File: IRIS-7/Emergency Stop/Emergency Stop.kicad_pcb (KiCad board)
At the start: 2 copper layers, 40 x 50 mm, 36 parts, among them IC1 LMR16006, J1 5mm TB, J2 ESTOP, J3 Pwr, J4 5mm TB, Q1 BSS123, Q2 BSS123, Q3 DMP3099L

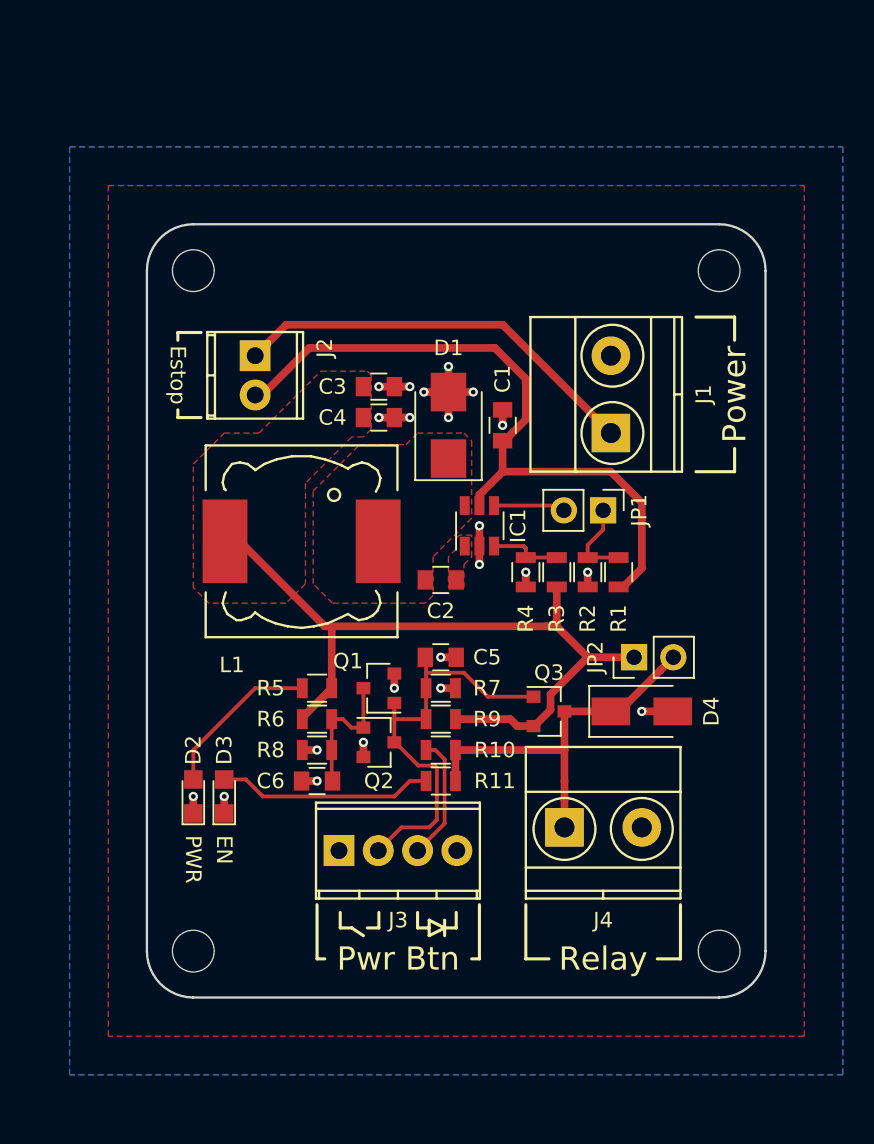
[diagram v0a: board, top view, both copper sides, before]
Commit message: Finalize board design for Rev A release
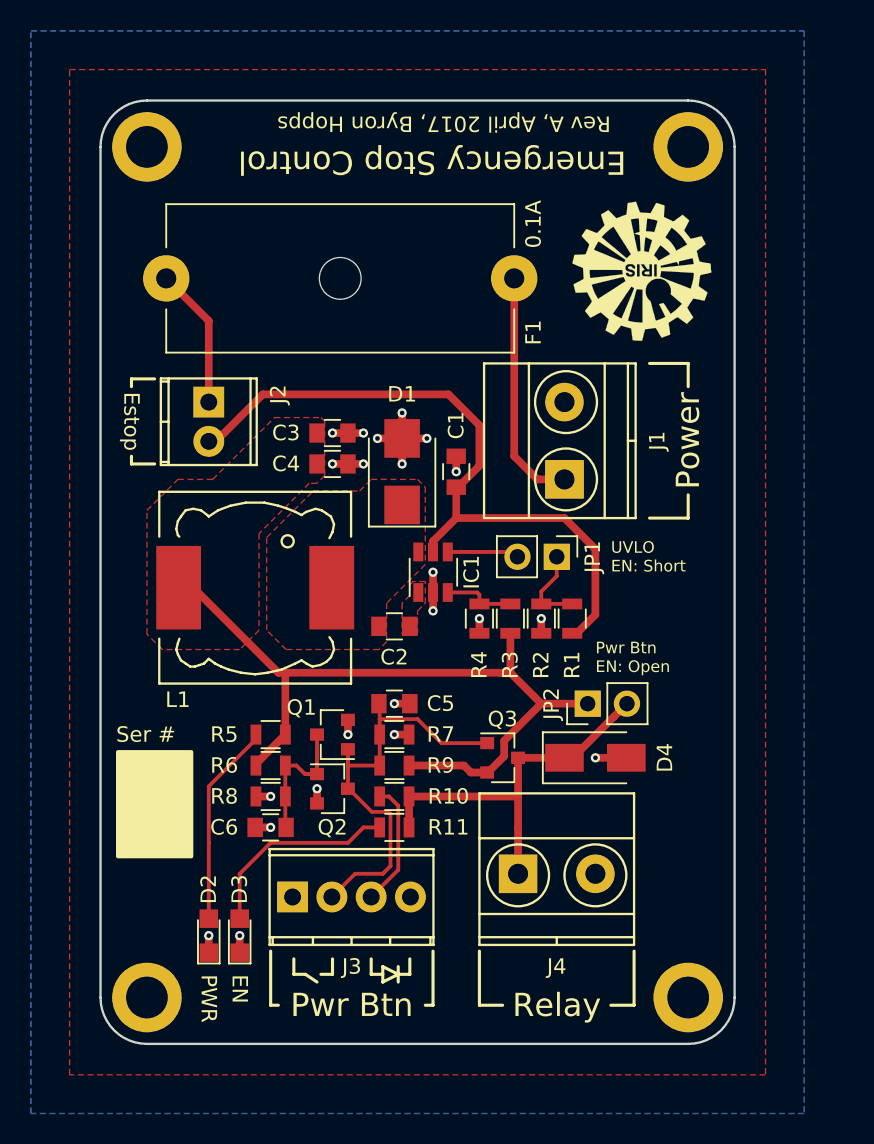
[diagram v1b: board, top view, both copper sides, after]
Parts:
- removed the REF** at (137.0, 97.0)
- removed the REF** at (103.0, 97.0)
- removed the REF** at (103.0, 53.0)
- removed the REF** at (137.0, 53.0)
- added F1: F, Fuse_Holders_and_Fuses:Fuseholder5x20_horiz_open_Schurter_0031_8201, F.Cu at (123.8, 53.5)
- added G***: LOGO, IRIS_Logos:IRIS_Logo_9.2, F.Cu at (132.0, 53.0)
- added REF**: MountingHole_2.7mm_M2.5_ISO7380_Pad, Mounting_Holes:MountingHole_2.7mm_M2.5_ISO7380_Pad, F.Cu at (100.0, 100.0)
- added REF**: MountingHole_2.7mm_M2.5_ISO7380_Pad, Mounting_Holes:MountingHole_2.7mm_M2.5_ISO7380_Pad, F.Cu at (135.0, 100.0)
- added REF**: MountingHole_2.7mm_M2.5_ISO7380_Pad, Mounting_Holes:MountingHole_2.7mm_M2.5_ISO7380_Pad, F.Cu at (135.0, 45.0)
- added REF**: MountingHole_2.7mm_M2.5_ISO7380_Pad, Mounting_Holes:MountingHole_2.7mm_M2.5_ISO7380_Pad, F.Cu at (100.0, 45.0)
- JP1, JP2: footprint Socket_Strips:Socket_Strip_Straight_1x02_Pitch2.54mm -> Pin_Headers:Pin_Header_Straight_1x02_Pitch2.54mm
- moved D2 9.06 mm to (104.0, 96.0)
- moved D3 9.06 mm to (106.0, 96.0)
- moved C1 4.24 mm to (120.0, 66.0)
- moved C2 4.24 mm to (116.0, 76.0)
- moved C3 4.24 mm to (112.0, 63.5)
- moved C4 4.24 mm to (112.0, 65.5)
- moved C5 4.24 mm to (116.0, 81.0)
- moved C6 4.24 mm to (108.0, 89.0)
- moved D1 4.24 mm to (116.5, 66.0)
- moved D4 4.24 mm to (129.0, 84.5)
- moved IC1 4.24 mm to (118.5, 72.5)
- moved J1 4.24 mm to (127.0, 66.5)
- moved J2 4.24 mm to (104.0, 61.5)
- moved J3 4.24 mm to (109.4, 93.5)
- moved J4 4.24 mm to (124.0, 92.0)
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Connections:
- J2 pad 1: /Vbatt -> /Vestop
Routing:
- net /Vbatt: track 26.7 -> 15.4 mm
- net /Vestop: track 0.00 -> 9.14 mm
- net Net-(D2-Pad2): track 10.6 -> 13.2 mm
- net Net-(D3-Pad2): track 14.2 -> 13.5 mm
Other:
- board size 40 x 50 mm -> 41 x 61 mm
- net class 0.5mm: clearance 0.2 -> 0.15
- net class Default: clearance 0.2 -> 0.15
- rule trace_clearance: 0.2 -> 0.15
- board text added: "0.1A"
- board text added: "Emergency Stop Control"
- board text added: "JP1 (UVLO)"
- board text added: "Notes"
- board text added: "Please place any manufacturing marks within this area"
- board text added: "Pwr Btn EN: Open"
- board text added: "Rev A, April 2017, Byron Hopps"
- board text added: "Ser #"
- board text added: "TH"
- board text added: "UVLO EN: Short"
- board text added: "V"
